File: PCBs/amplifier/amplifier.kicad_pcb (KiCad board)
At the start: 2 copper layers, 200 x 100 mm, 99 parts, among them J1 6V3A, J10 LS1A, J2 6V3B, J3 AUX-IN, J4 AUX-IN-GND, J5 +38V, J6 -38V, J7 GND, J8 +310V, J9 LS1B, P1 2k, P2 5k, P3 5k, Q1 BD139, Q10 BC547, Q2 2SC2073, Q3 2SA940, Q4 2SC5200, Q5 2SC5200, Q6 BC550, Q7 BC550, Q8 BS170, Q9 BC547, U1 LM337, U2 LM317

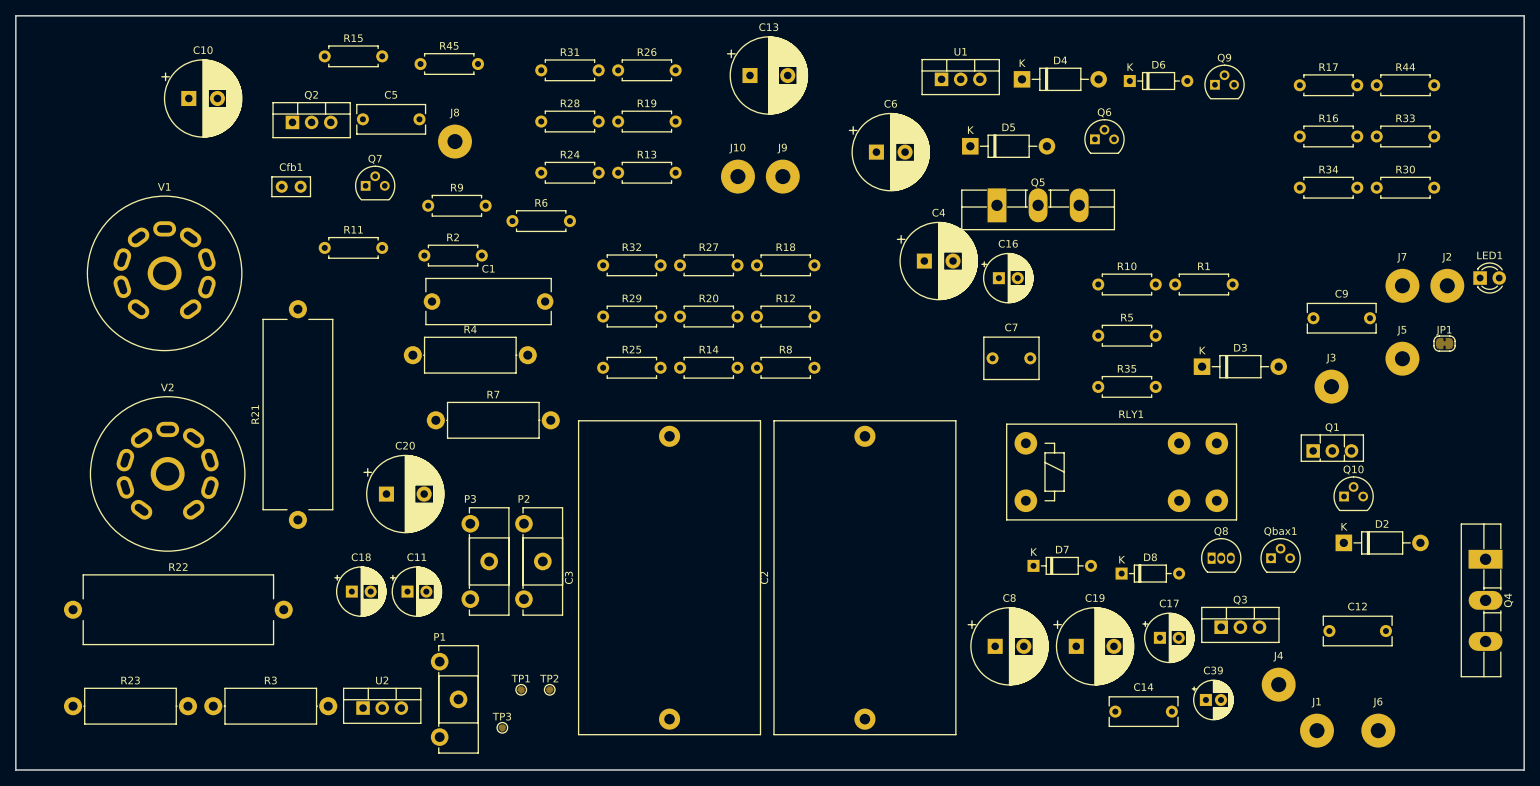
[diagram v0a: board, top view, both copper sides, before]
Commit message: Rough component placement amp. pcb.
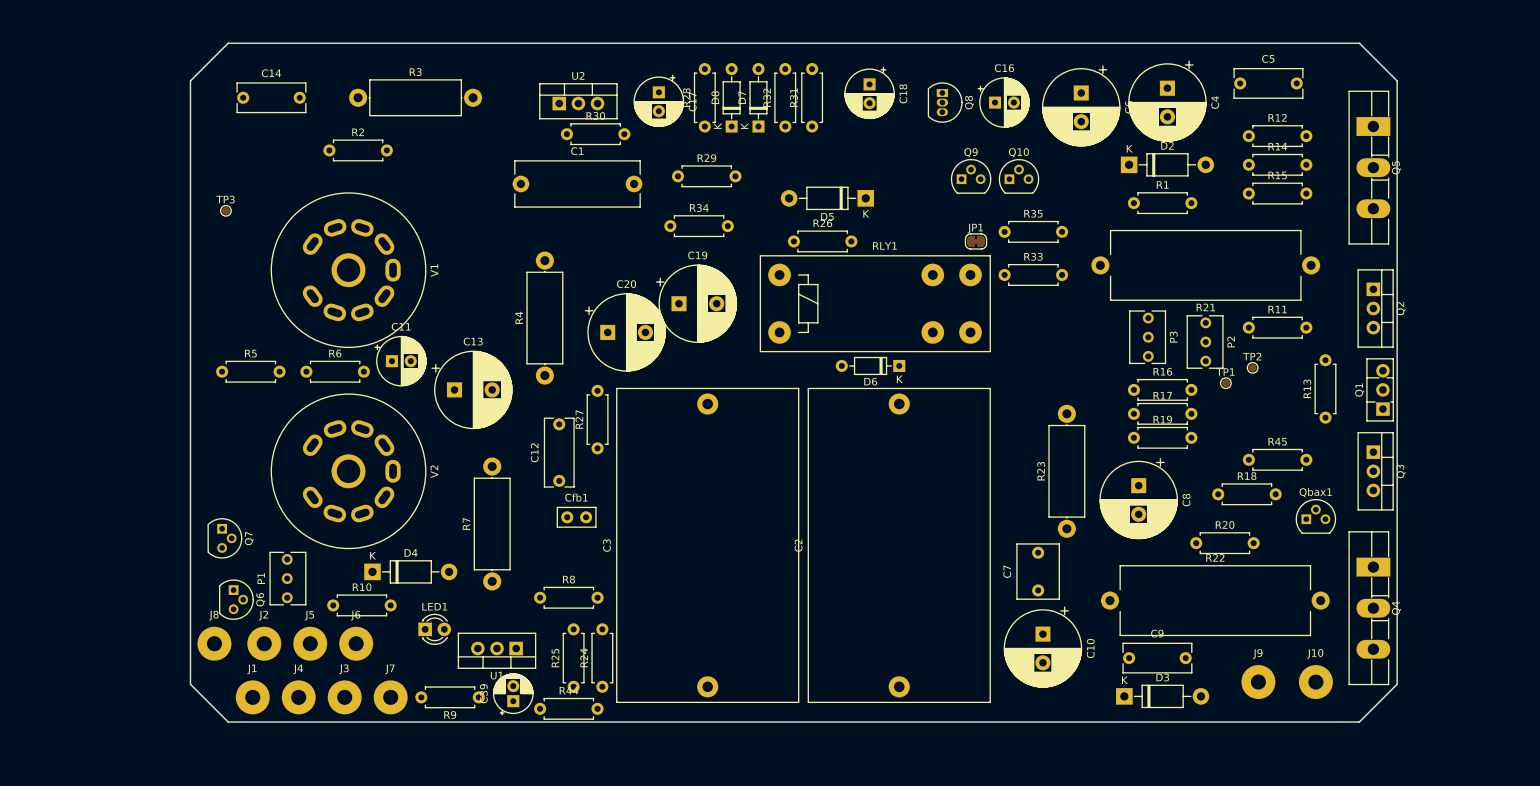
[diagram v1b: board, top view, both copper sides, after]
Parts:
- P1, P2, P3: footprint Potentiometer_THT:Potentiometer_ACP_CA14-H2,5_Horizontal -> Potentiometer_THT:Potentiometer_Bourns_3266Y_Vertical
- moved J2 163.9 mm to (74.8, 124.6)
- moved J5 149.7 mm to (80.9, 124.6)
- moved LED1 147.4 mm to (96.1, 122.7)
- moved Q2 145.0 mm to (221.8, 77.6), turned to 270 degrees
- moved J7 144.8 mm to (91.5, 131.7)
- moved C14 141.4 mm to (72.0, 52.2)
- moved J1 141.2 mm to (73.3, 131.7)
- moved R21 138.5 mm to (213.6, 74.5), turned to 180 degrees
- moved R44 138.4 mm to (111.4, 133.3)
- moved R22 137.5 mm to (186.9, 118.9)
- moved J3 137.2 mm to (85.5, 131.7)
- moved J6 136.0 mm to (87.0, 124.6)
- moved R23 133.9 mm to (181.2, 109.4), turned to 90 degrees
- moved C10 133.7 mm to (178.0, 123.3), turned to 270 degrees
- moved J4 130.0 mm to (79.4, 131.7)
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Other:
- board size 200 x 100 mm -> 160 x 90 mm
